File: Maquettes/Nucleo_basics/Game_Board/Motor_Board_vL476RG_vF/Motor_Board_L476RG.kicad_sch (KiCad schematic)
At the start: 43 parts, among them CON1 MikroE-Accelero, CON2 MikroE-nRF-S-module, J1 Speed_R, J10 Morpho_Gauche, J11 Morpho_Droite, J12 LED_1, J13 LED_2, J14 LED_3, J15 LED_4, J17 I2C_Visu, J18 I2C_EXT, J19 GND_reg, J2 Speed_L, J20 3.3V_reg, J21 MOT_R, J22 MOT_L, J23 D_IN_OUT, J3 Line_R, J4 Line_C, J5 Line_L, J6 US_Sensor, J7 Servo, J8 BAT_IN, J9 TC74A2-TempI2C, SW1 SW_1, SW2 SW_2, U1 MCP9700-Temp, U2 LM7805_TO220, U3 SN754410NE

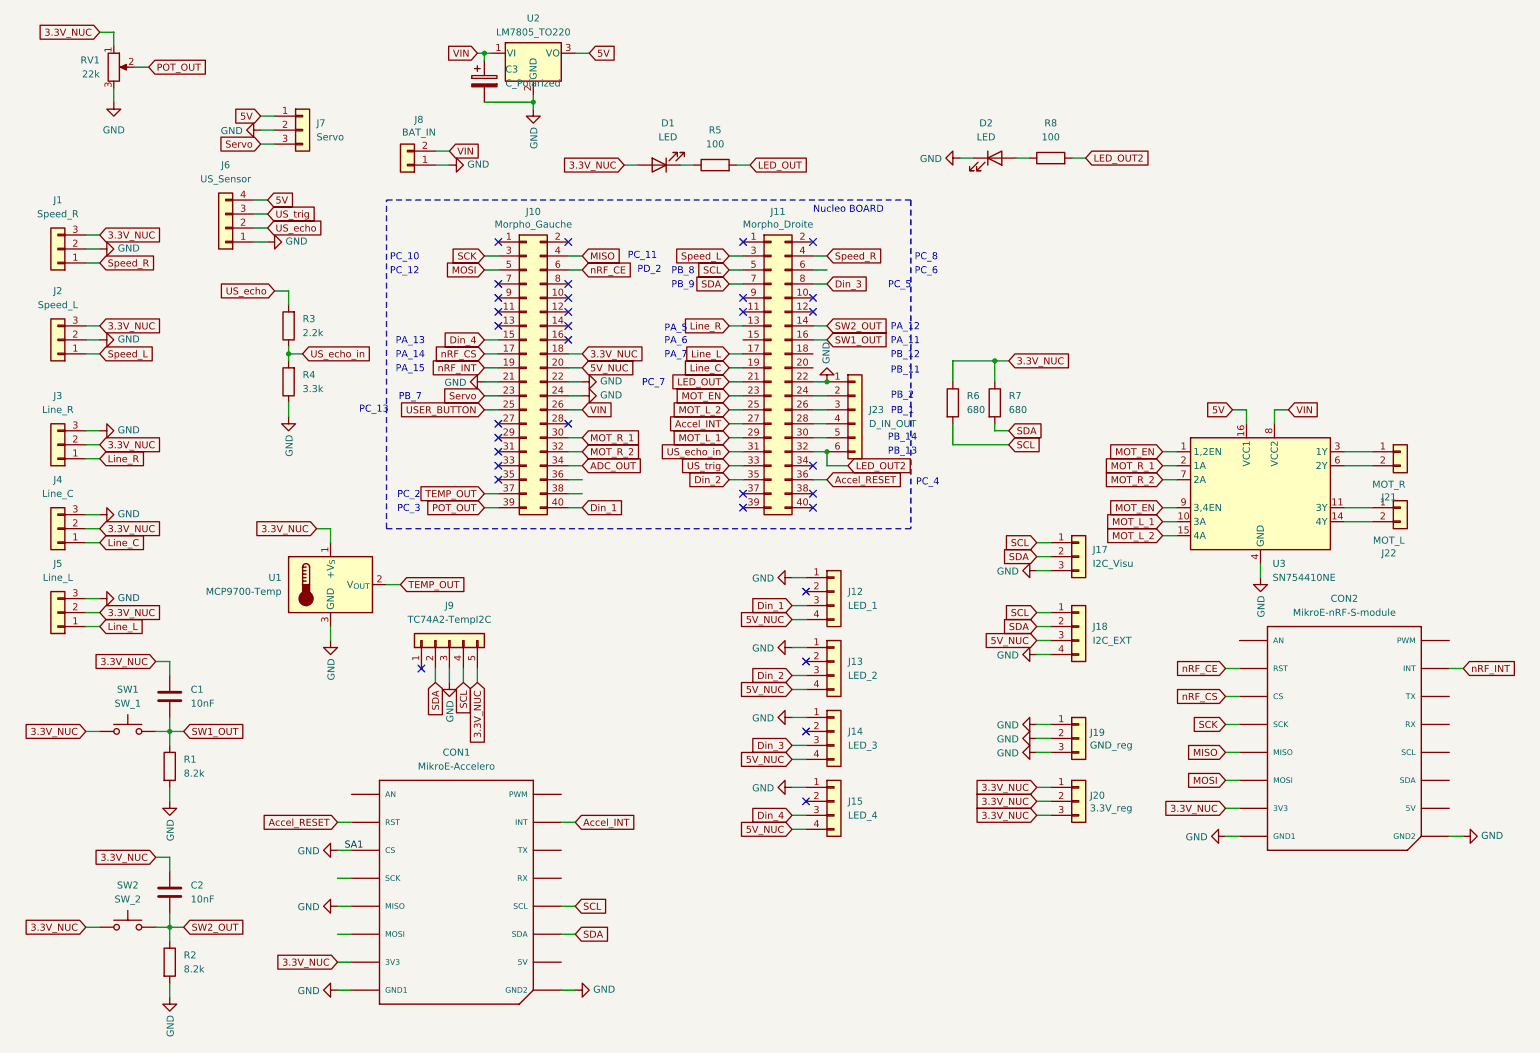
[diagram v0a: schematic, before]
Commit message: Update Robot Board
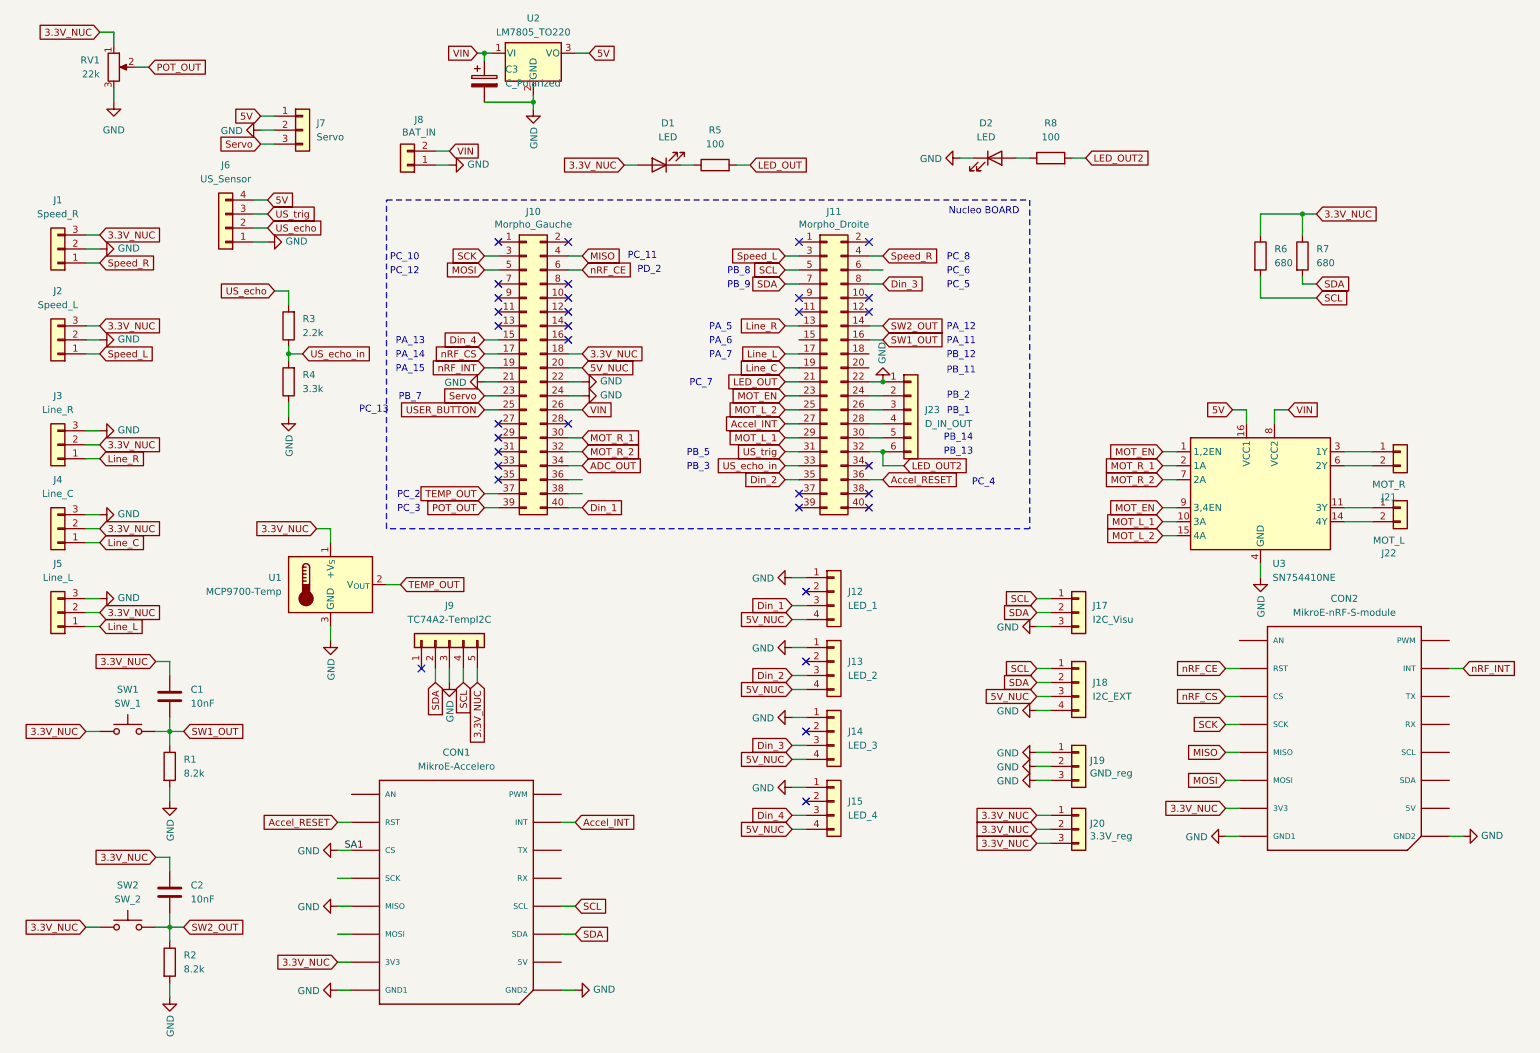
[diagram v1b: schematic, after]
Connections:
- net US_echo_in: now also J11.33 (Pin_33); no longer J11.31 (Pin_31)
- net US_trig: now also J11.31 (Pin_31); no longer J11.33 (Pin_33)
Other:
- note added: "PB_3"
- note added: "PB_5"
- moved on the sheet: J11, J17, J18, J19, J20, J23, R6, R7
